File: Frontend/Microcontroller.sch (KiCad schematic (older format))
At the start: 57 parts, among them J10 SWD, Q1 ULN2003AD, U17 MAX5725AAUP, U18 STM32F030C8T

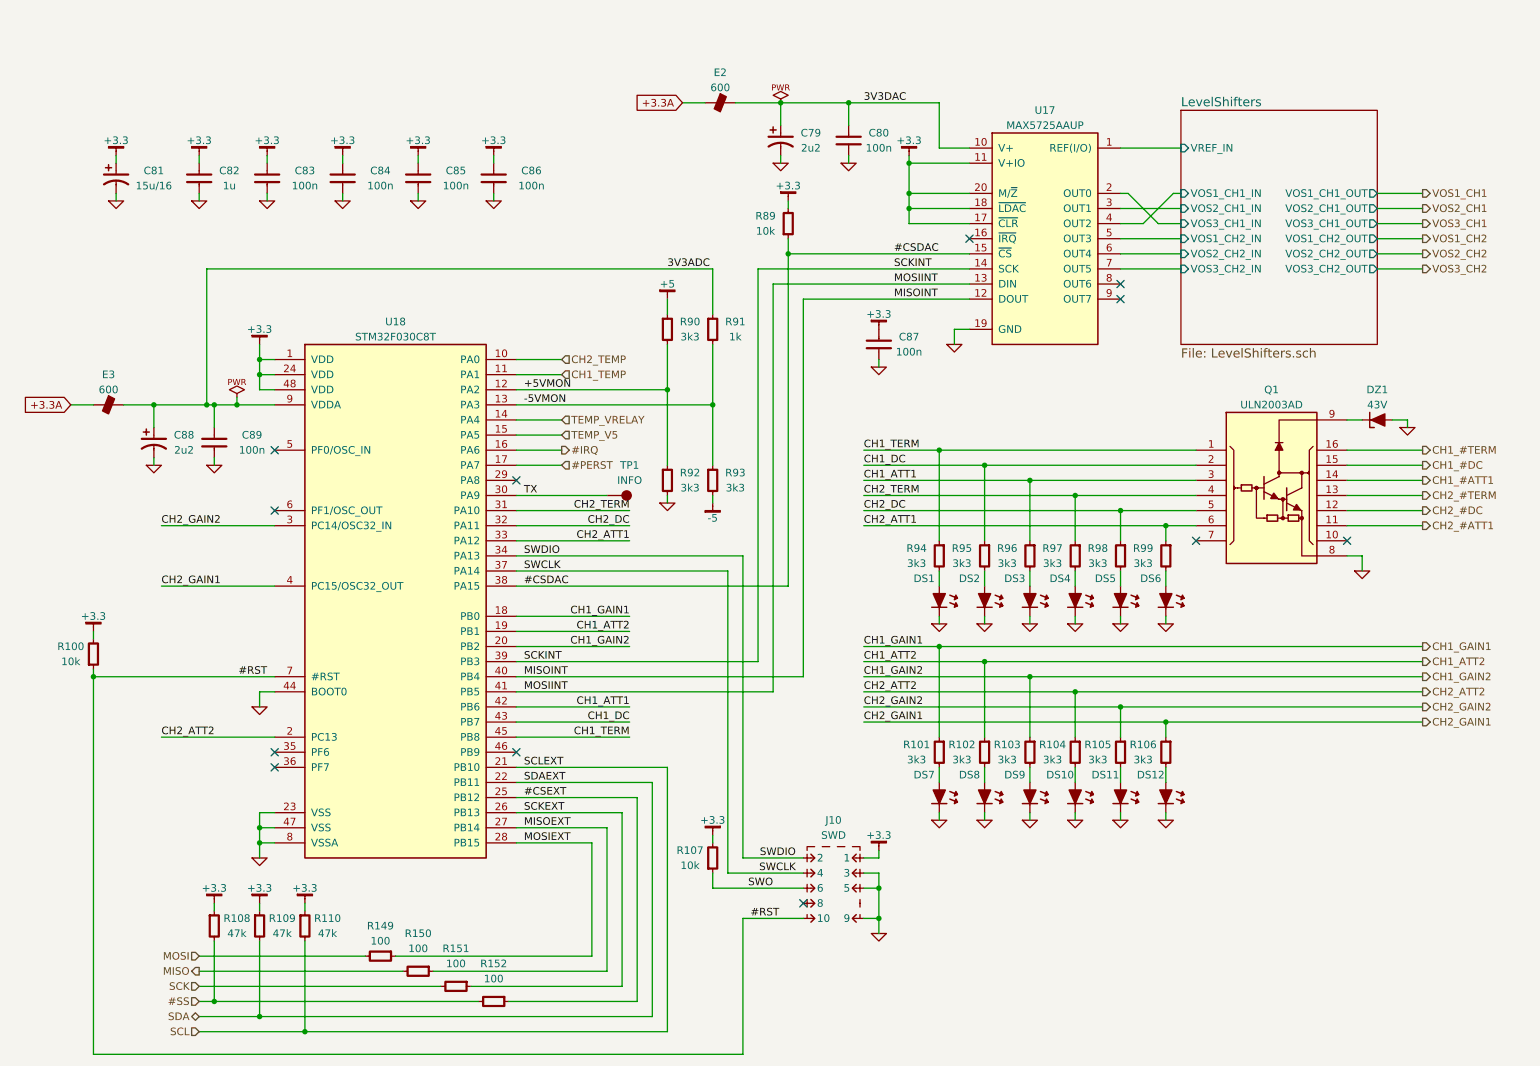
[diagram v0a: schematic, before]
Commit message: Schematic cleanup
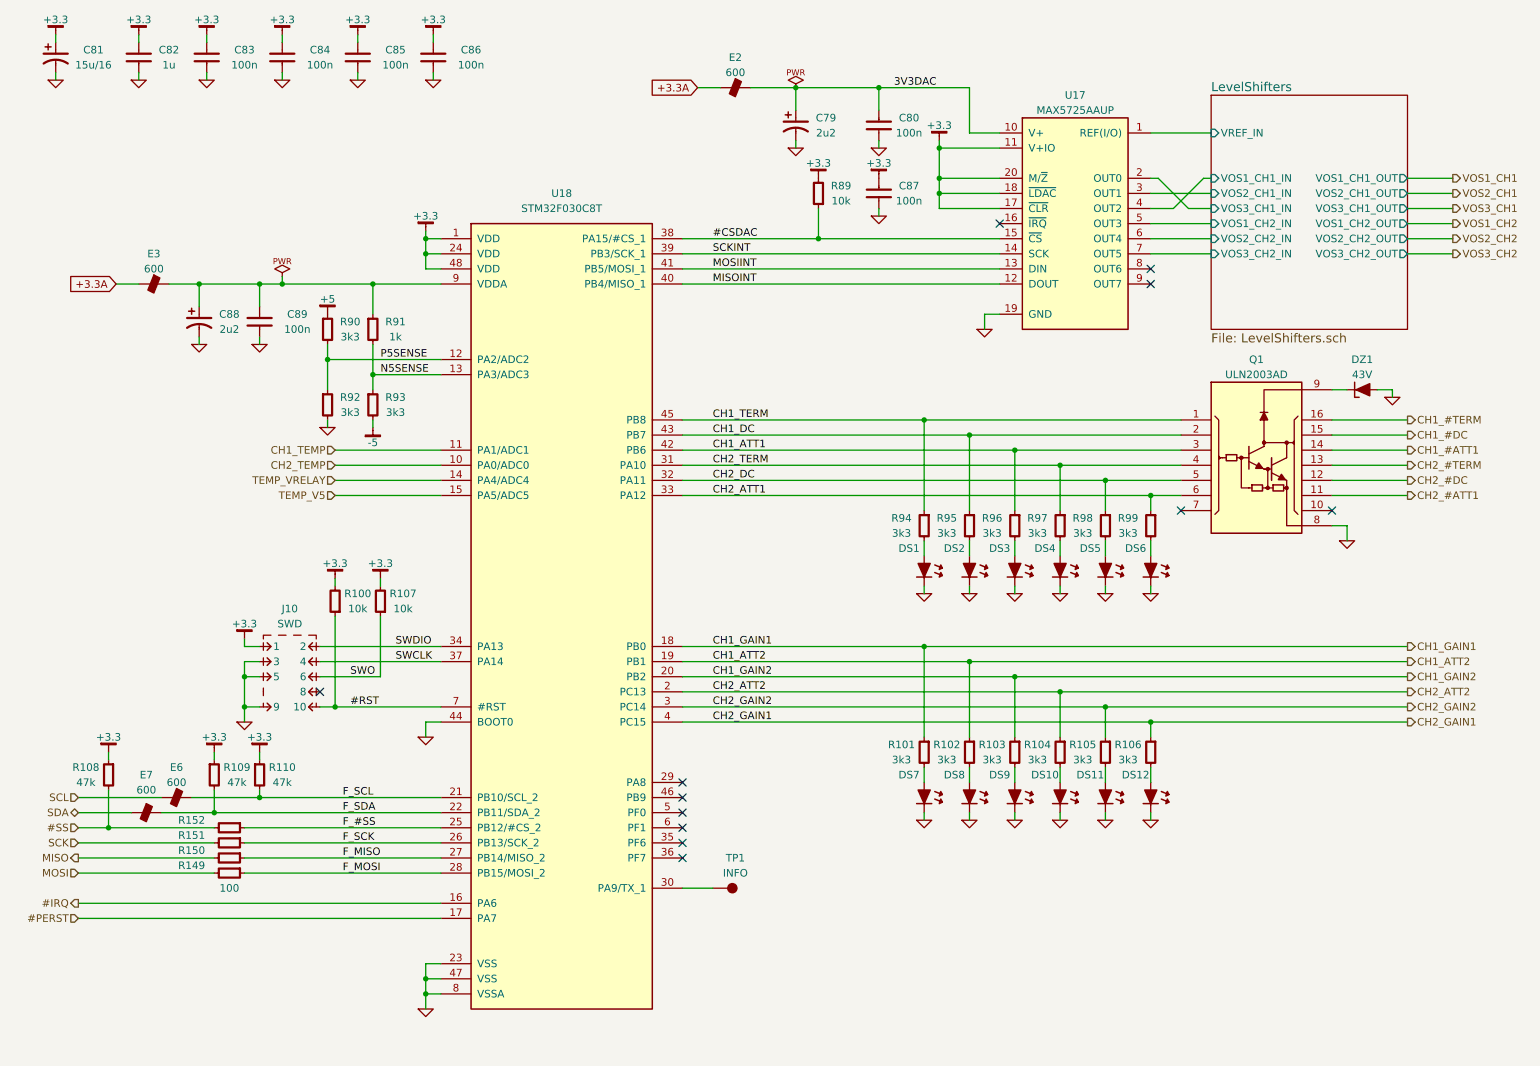
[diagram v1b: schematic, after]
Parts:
- removed U18: STM32F030C8T, IPC7351-Nominal:QFP50P900X900X160-48, symbol STM32F030x4,6,8-LQFP48
- added E6, E7: 600, IPC7351-Nominal:INDC1005X60, symbol BEAD-0402
- added U18: STM32F030C8T, IPC7351-Nominal:QFP50P900X900X160-48, symbol STM32F030x4,6,8-LQFP48-OSFE
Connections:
- net #CSDAC: now also U18.38 (PA15/#CS_1)
- net #IRQ: now also U18.16 (PA6)
- net #PERST: now also U18.17 (PA7)
- net #RST: now also U18.7 (#RST)
- net +3.3: now also U18.1 (VDD), U18.24 (VDD), U18.48 (VDD)
- net CH1_ATT1: now also U18.42 (PB6)
- net CH1_ATT2: now also U18.19 (PB1)
- net CH1_DC: now also U18.43 (PB7)
- net CH1_GAIN1: now also U18.18 (PB0)
- net CH1_GAIN2: now also U18.20 (PB2)
- net CH1_TEMP: now also U18.11 (PA1/ADC1)
- net CH1_TERM: now also U18.45 (PB8)
- net CH2_ATT1: now also U18.33 (PA12)
- net CH2_ATT2: now also U18.2 (PC13)
- net CH2_DC: now also U18.32 (PA11)
- net CH2_GAIN1: now also U18.4 (PC15)
- net CH2_GAIN2: now also U18.3 (PC14)
- net CH2_TEMP: now also U18.10 (PA0/ADC0)
- net CH2_TERM: now also U18.31 (PA10)
- net GND: now also U18.23 (VSS), U18.44 (BOOT0), U18.47 (VSS), U18.8 (VSSA)
- net MISOINT: now also U18.40 (PB4/MISO_1)
- net MOSIINT: now also U18.41 (PB5/MOSI_1)
- net SCKINT: now also U18.39 (PB3/SCK_1)
- net SCL: now also E6.1; no longer R110.2
- net SDA: now also E7.1; no longer R109.2
- net SWCLK: now also U18.37 (PA14)
- net SWDIO: now also U18.34 (PA13)
- net TEMP_V5: now also U18.15 (PA5/ADC5)
- net TEMP_VRELAY: now also U18.14 (PA4/ADC4)
- net #CSEXT renamed F_#SS
- net F_#SS: now also U18.25 (PB12/#CS_2)
- net +5VMON renamed P5SENSE
- net P5SENSE: now also U18.12 (PA2/ADC2)
- net -5VMON renamed N5SENSE
- net N5SENSE: now also U18.13 (PA3/ADC3)
- net 3V3ADC: no longer names the net of C88.1, C89.1, E3.2, R91.1
- net 3V3ADC: now also U18.9 (VDDA)
- net MISOEXT renamed F_MISO
- net F_MISO: now also U18.27 (PB14/MISO_2)
- net MOSIEXT renamed F_MOSI
- net F_MOSI: now also U18.28 (PB15/MOSI_2)
- net SCKEXT renamed F_SCK
- net F_SCK: now also U18.26 (PB13/SCK_2)
- net TX: no longer names the net of TP1.1
- net TX: now also U18.30 (PA9/TX_1)
- new net F_SCL: E6.2, R110.2, U18.21 (PB10/SCL_2)
- new net F_SDA: E7.2, R109.2, U18.22 (PB11/SDA_2)
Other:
- moved on the sheet: C79, C80, C81, C82, C83, C84, C85, C86, C87, C88, C89, DS1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
